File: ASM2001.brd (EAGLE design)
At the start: 22.5 x 21.3 mm, 25 parts, among them J1 3013, J2 DF12-32-DP, J3 961102, J4 SM02B-SRSS-TB(LF)(SN), Q2 DMP2035U, SW1 PCM12SMTR, U1 ATMEGA328P, U2 MCP73831, Y1 8.00MHZ

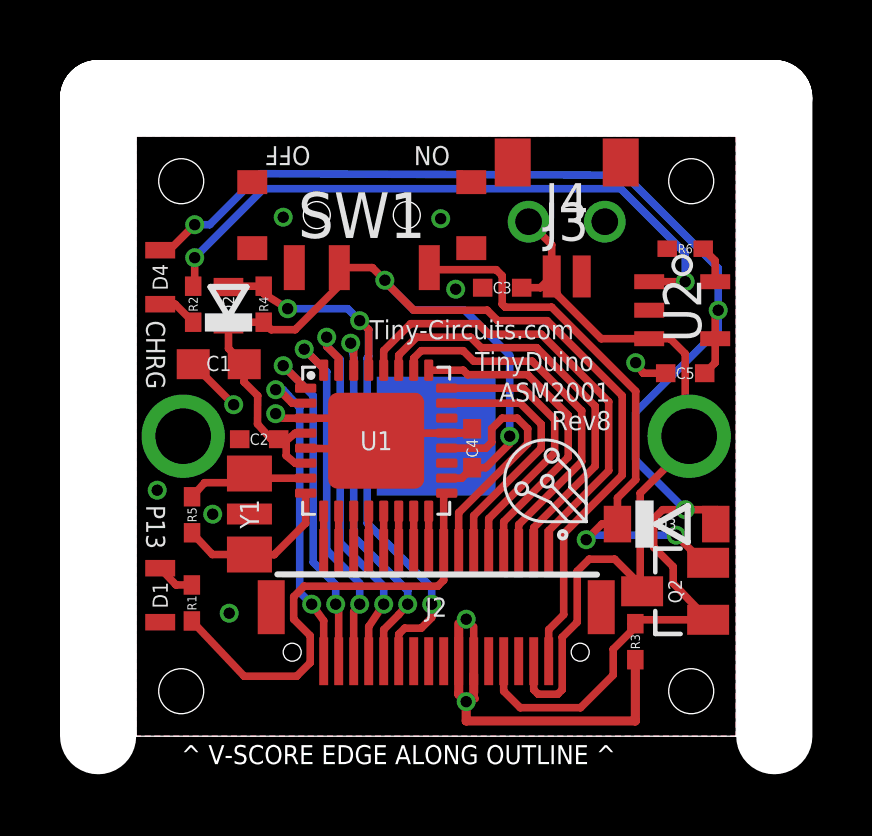
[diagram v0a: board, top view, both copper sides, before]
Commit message: Update to Rev 9
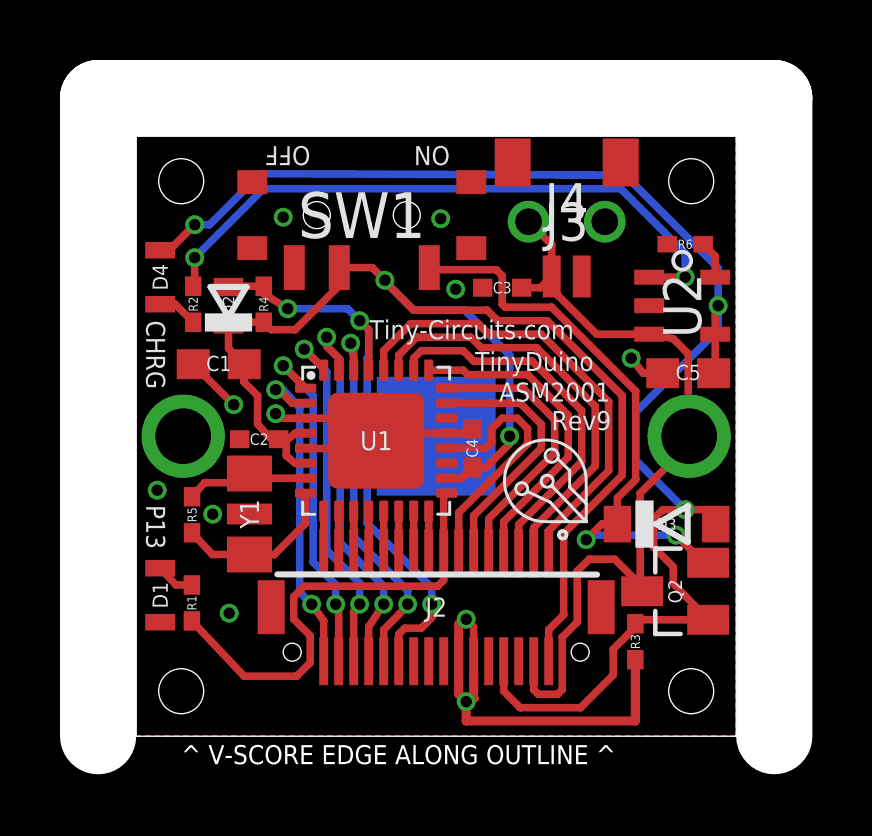
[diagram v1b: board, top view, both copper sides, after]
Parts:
- C5: value 4.7uF -> 10uF; device tinycircuits:C0402 -> tinycircuits:C0603
- moved U2 0.15 mm to (28.2, 24.4)
- moved R6 0.15 mm to (28.3, 26.4)
- moved C5 0.10 mm to (28.4, 22.1)
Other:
- board text added: "9"
- board text added: "Rev9"
- board text removed: "8"
- board text removed: "Rev8"
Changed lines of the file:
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@@
 <text x="48.111025" y="4.365003125" size="0.889" layer="48">TinyDuino - 20mm</text>
 <text x="44.986825" y="1.7714" size="0.889" layer="48">AS-PCB-ASM2001</text>
-<text x="67.3810375" y="1.6952" size="0.889" layer="48">8</text>
+<text x="67.3810375" y="1.6952" size="0.889" layer="48">9</text>
 <wire x1="10" y1="30" x2="30" y2="30" width="0.0254" layer="20"/>
 <wire x1="30" y1="30" x2="30" y2="10" width="0.0254" layer="20"/>
@@
 <wire x1="10.1778" y1="10.1778" x2="29.8222" y2="10.1778" width="0.3556" layer="42"/>
 <text x="11.5" y="9.0678" size="0.635" layer="20">^ V-SCORE EDGE ALONG OUTLINE ^</text>
-<text x="23.84581875" y="20.203640625" size="0.635" layer="21">Rev8</text>
+<text x="23.84581875" y="20.203640625" size="0.635" layer="21">Rev9</text>
 <text x="14.05924375" y="29.6694" size="0.635" layer="22" rot="MR180">OFF</text>
 <text x="19.30924375" y="29.6694" size="0.635" layer="22" rot="MR180">ON</text>
@@
 <attribute name="VALUE" value="961102" x="24.35" y="27.15" size="1.778" layer="27" display="off"/>
 </element>
-<element name="U2" library="tinycircuits" package="SOT-23" value="MCP73831 " x="28.2" y="24.2" rot="R270">
-<attribute name="PARTNO" value="AS-ITM-00136" x="28.2" y="24.2" size="1.778" layer="27" rot="R270" display="off"/>
-<attribute name="VALUE" value="MCP73831 " x="28.2" y="24.2" size="1.778" layer="27" rot="R270" display="off"/>
+<element name="U2" library="tinycircuits" package="SOT-23" value="MCP73831 " x="28.2" y="24.35" rot="R270">
+<attribute name="PARTNO" value="AS-ITM-00136" x="28.2" y="24.35" size="1.778" layer="27" rot="R270" display="off"/>
+<attribute name="VALUE" value="MCP73831 " x="28.2" y="24.35" size="1.778" layer="27" rot="R270" display="off"/>
 </element>
-<element name="R6" library="tinycircuits" package="0402" value="10K" x="28.3" y="26.25" rot="R180">
-<attribute name="VALUE" value="10.0K" x="28.3" y="26.25" size="1.778" layer="27" rot="R180" display="off"/>
-<attribute name="PARTNO" value="AS-ITM-00032" x="28.3" y="26.25" size="1.778" layer="27" rot="R180" display="off"/>
+<element name="R6" library="tinycircuits" package="0402" value="10K" x="28.3" y="26.4" rot="R180">
+<attribute name="VALUE" value="10.0K" x="28.3" y="26.4" size="1.778" layer="27" rot="R180" display="off"/>
+<attribute name="PARTNO" value="AS-ITM-00032" x="28.3" y="26.4" size="1.778" layer="27" rot="R180" display="off"/>
 </element>
 <element name="J4" library="tinycircuits" package="JST_SH_2X1" value="SM02B-SRSS-TB(LF)(SN)" x="24.35" y="27.8" rot="R180">
@@
 <attribute name="VALUE" value="SM02B-SRSS-TB(LF)(SN)" x="24.35" y="27.8" size="1.778" layer="27" rot="R180" display="off"/>
 </element>
-<element name="C5" library="tinycircuits" package="C0402" value="4.7uF" x="28.3" y="22.1" rot="R180">
-<attribute name="PARTNO" value="AS-ITM-00242" x="28.3" y="22.1" size="1.778" layer="27" rot="R180" display="off"/>
-<attribute name="VALUE" value="4.7uF" x="28.3" y="22.1" size="1.778" layer="27" rot="R180" display="off"/>
-<attribute name="DATABASE" value="./../../../../../Components/TinyCircuits_Part_Database.txt" x="28.3" y="22.1" size="1.778" layer="27" rot="R180" display="off"/>
+<element name="C5" library="tinycircuits" package="C0603" value="10uF" x="28.4" y="22.1" rot="R180">
+<attribute name="PARTNO" value="AS-ITM-00002" x="28.4" y="22.1" size="1.778" layer="27" rot="R180" display="off"/>
+<attribute name="VALUE" value="10uF" x="28.4" y="22.1" size="1.778" layer="27" rot="R180" display="off"/>
+<attribute name="DATABASE" value="./../../../../../Components/TinyCircuits_Part_Database.txt" x="28.4" y="22.1" size="1.778" layer="27" rot="R180" display="off"/>
 </element>
 <element name="D4" library="tinycircuits" package="LNJ_LED" value="AMBER" x="10.8" y="25.3">
@@
 <via x="20.15" y="27.25" extent="1-16" drill="0.381"/>
 <via x="14.9" y="27.3" extent="1-16" drill="0.381"/>
-<via x="26.65" y="22.45" extent="1-16" drill="0.381"/>
+<via x="26.5" y="22.6" extent="1-16" drill="0.381"/>
 <wire x1="21.25" y1="12.05" x2="21.25" y2="11.45" width="0.3048" layer="1"/>
 <wire x1="20.75" y1="11.4" x2="20.75" y2="13.75" width="0.3048" layer="1"/>
@@
 <wire x1="20.3508" y1="20.1" x2="21.1" y2="20.1" width="0.254" layer="1"/>
 <wire x1="21.1" y1="20.1" x2="21.2" y2="20.25" width="0.254" layer="1"/>
-<wire x1="27.65" y1="22.1" x2="26.9" y2="22.1" width="0.254" layer="1"/>
-<wire x1="26.9" y1="22.1" x2="26.65" y2="22.45" width="0.254" layer="1"/>
+<wire x1="27.55" y1="22.1" x2="26.9" y2="22.1" width="0.254" layer="1"/>
+<wire x1="26.9" y1="22.1" x2="26.5" y2="22.6" width="0.254" layer="1"/>
 <wire x1="15.6492" y1="20.6" x2="14.7992" y2="20.6" width="0.254" layer="1"/>
 <wire x1="14.7992" y1="20.6" x2="14.65" y2="20.75" width="0.254" layer="1"/>
@@
 <contactref element="J4" pad="2"/>
 <wire x1="23.85" y1="25.325" x2="24.05" y2="24.7" width="0.254" layer="1"/>
-<wire x1="24.05" y1="24.7" x2="25.5" y2="23.25" width="0.254" layer="1"/>
-<wire x1="25.5" y1="23.25" x2="27.1" y2="23.25" width="0.254" layer="1"/>
-<wire x1="28.4328" y1="20" x2="28.3" y2="20.1328" width="0.254" layer="1"/>
-<wire x1="28.3" y1="20.1328" x2="28.3" y2="22.75" width="0.254" layer="1"/>
-<wire x1="28.3" y1="22.75" x2="27.8" y2="23.25" width="0.254" layer="1"/>
-<wire x1="27.8" y1="23.25" x2="27.1" y2="23.25" width="0.254" layer="1"/>
+<wire x1="24.05" y1="24.7" x2="25.35" y2="23.4" width="0.254" layer="1"/>
+<wire x1="25.35" y1="23.4" x2="27.1" y2="23.4" width="0.254" layer="1"/>
+<wire x1="28.4328" y1="20" x2="28.4" y2="20.1328" width="0.254" layer="1"/>
+<wire x1="28.4" y1="20.1328" x2="28.4" y2="22.75" width="0.254" layer="1"/>
+<wire x1="28.4" y1="22.75" x2="27.9" y2="23.25" width="0.254" layer="1"/>
+<wire x1="27.9" y1="23.25" x2="27.1" y2="23.4" width="0.254" layer="1"/>
 <wire x1="23.85" y1="25.325" x2="23.85" y2="26.38" width="0.254" layer="1"/>
 <wire x1="23.25" y1="12.4999" x2="23.25" y2="11.55" width="0.254" layer="1"/>
@@
 <wire x1="26.65" y1="19.2" x2="26.65" y2="20.8" width="0.254" layer="16"/>
 <wire x1="26.65" y1="20.8" x2="29.4" y2="23.55" width="0.254" layer="16"/>
-<wire x1="29.4" y1="23.55" x2="29.4" y2="24.2" width="0.254" layer="16"/>
-<via x="29.4" y="24.2" extent="1-16" drill="0.381"/>
+<wire x1="29.4" y1="23.55" x2="29.4" y2="24.35" width="0.254" layer="16"/>
+<via x="29.4" y="24.35" extent="1-16" drill="0.381"/>
 <contactref element="C5" pad="1"/>
-<wire x1="29.3" y1="23.25" x2="29.3" y2="24.1" width="0.254" layer="1"/>
-<wire x1="29.3" y1="24.1" x2="29.4" y2="24.2" width="0.254" layer="1"/>
-<wire x1="29.3" y1="23.25" x2="29.3" y2="22.45" width="0.254" layer="1"/>
-<wire x1="29.3" y1="22.45" x2="28.95" y2="22.1" width="0.254" layer="1"/>
+<wire x1="29.3" y1="23.4" x2="29.3" y2="24.25" width="0.254" layer="1"/>
+<wire x1="29.3" y1="24.25" x2="29.4" y2="24.35" width="0.254" layer="1"/>
+<wire x1="29.3" y1="23.4" x2="29.3" y2="22.45" width="0.254" layer="1"/>
+<wire x1="29.3" y1="22.45" x2="29.25" y2="22.1" width="0.254" layer="1"/>
 <wire x1="22.25" y1="12.4999" x2="22.25" y2="11.5" width="0.254" layer="1"/>
 <wire x1="22.25" y1="11.5" x2="22.8" y2="10.95" width="0.254" layer="1"/>
@@
 <wire x1="14.15" y1="28.75" x2="26.3" y2="28.7" width="0.254" layer="16"/>
 <wire x1="26.3" y1="28.7" x2="29.4" y2="25.6" width="0.254" layer="16"/>
-<wire x1="29.4" y1="25.6" x2="29.4" y2="24.2" width="0.254" layer="16"/>
+<wire x1="29.4" y1="25.6" x2="29.4" y2="24.35" width="0.254" layer="16"/>
 </signal>
 <signal name="VCC">
@@
 <contactref element="U2" pad="5"/>
 <contactref element="R6" pad="1"/>
-<wire x1="29.3" y1="25.15" x2="29.3" y2="25.85" width="0.254" layer="1"/>
-<wire x1="29.3" y1="25.85" x2="28.9" y2="26.25" width="0.254" layer="1"/>
+<wire x1="29.3" y1="25.3" x2="29.3" y2="26" width="0.254" layer="1"/>
+<wire x1="29.3" y1="26" x2="28.9" y2="26.4" width="0.254" layer="1"/>
 </signal>
 <signal name="N$7">
@@
 <wire x1="14.25" y1="28.25" x2="26.15" y2="28.25" width="0.254" layer="16"/>
 <wire x1="26.15" y1="28.25" x2="28.3" y2="26.1" width="0.254" layer="16"/>
-<wire x1="28.3" y1="26.1" x2="28.3" y2="25.15" width="0.254" layer="16"/>
-<via x="28.3" y="25.15" extent="1-16" drill="0.381"/>
-<wire x1="28.3" y1="25.15" x2="27.1" y2="25.15" width="0.254" layer="1"/>
+<wire x1="28.3" y1="26.1" x2="28.3" y2="25.3" width="0.254" layer="16"/>
+<via x="28.3" y="25.3" extent="1-16" drill="0.381"/>
+<wire x1="28.3" y1="25.3" x2="27.1" y2="25.3" width="0.254" layer="1"/>
 </signal>
 <signal name="N$5">
